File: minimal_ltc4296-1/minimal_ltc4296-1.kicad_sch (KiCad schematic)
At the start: 44 parts, among them J1 TBP02R1-381-03BE, J2 TBP02R1-381-03BE, J3 TBP02R1-381-03BE, J4 TBP02R1-381-03BE, J5 TBP02R1-381-03BE, J6 TBP02R1-381-02BE, Q1 100.0 V, Q2 100.0 V, Q3 100.0 V, Q4 100.0 V, Q5 100.0 V, Q6 100.0 V, U1 LTC4296AUK-1-PBF

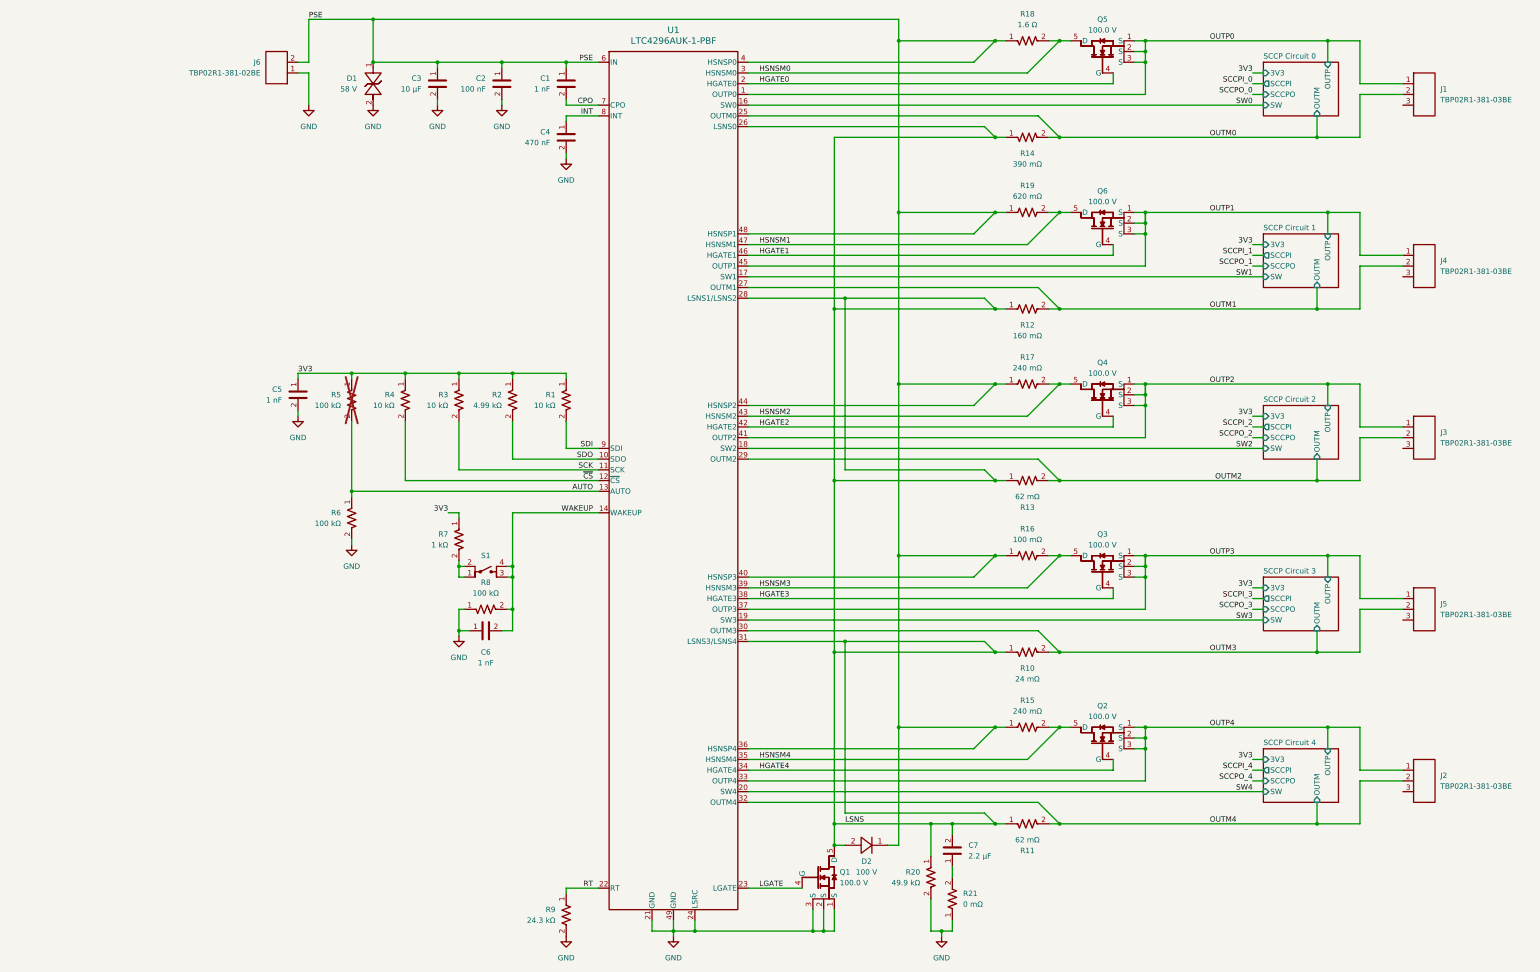
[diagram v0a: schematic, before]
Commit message: Update KiCad PCB file
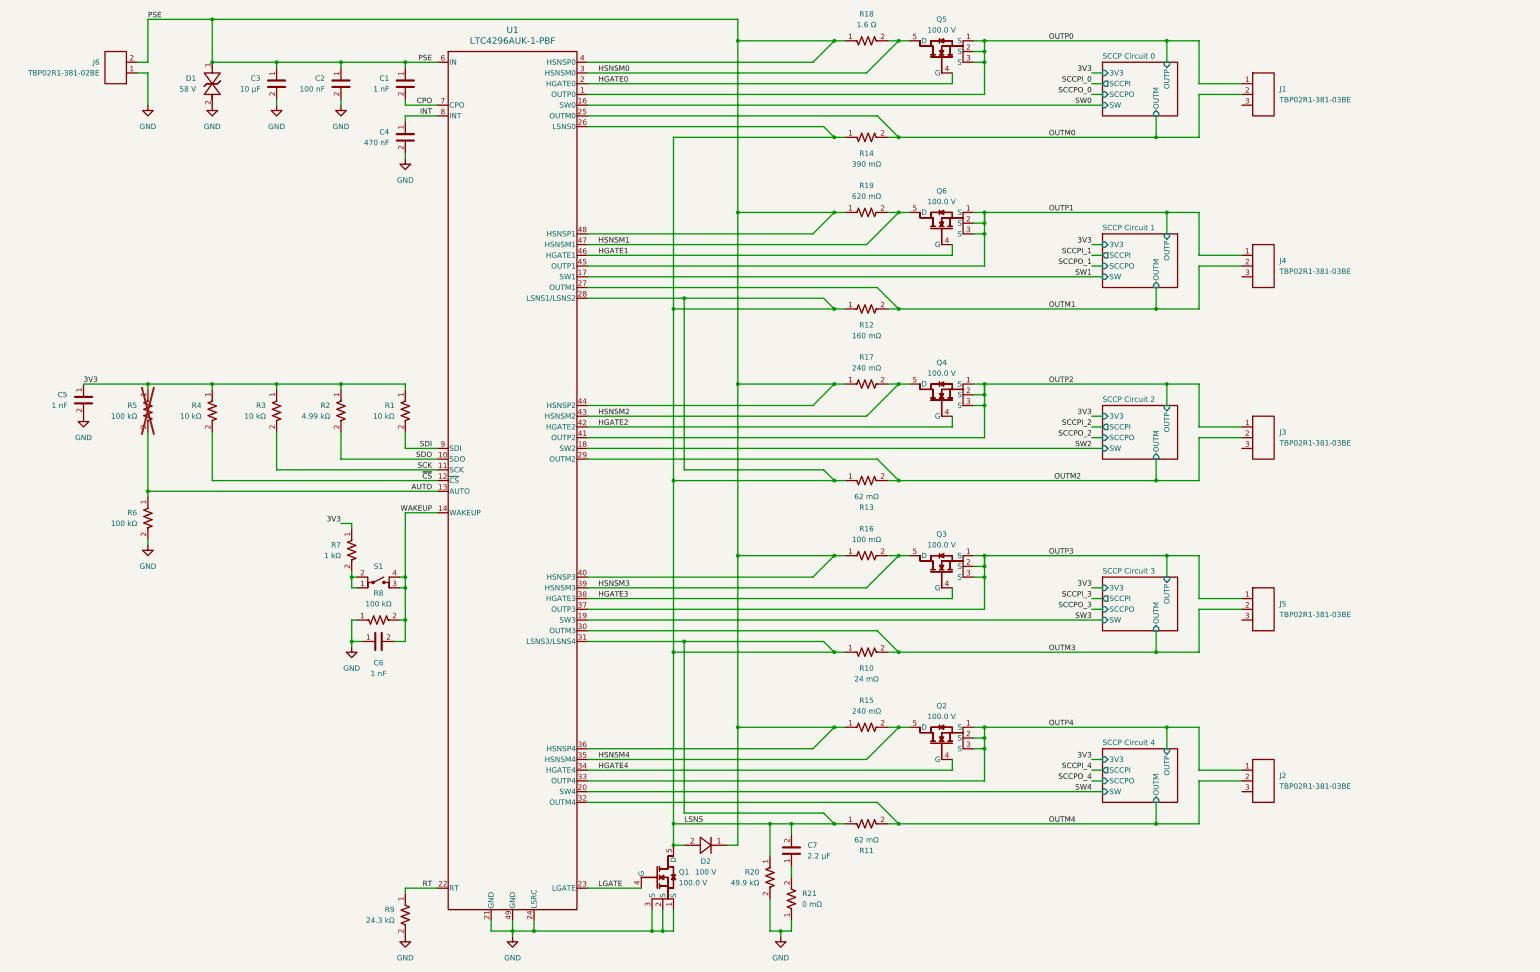
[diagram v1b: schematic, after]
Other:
- moved on the sheet: C1, C2, C3, C4, C5, C6, C7, D1, D2, J1, J2, J3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
